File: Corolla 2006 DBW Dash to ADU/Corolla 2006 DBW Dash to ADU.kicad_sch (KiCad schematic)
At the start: 5 parts

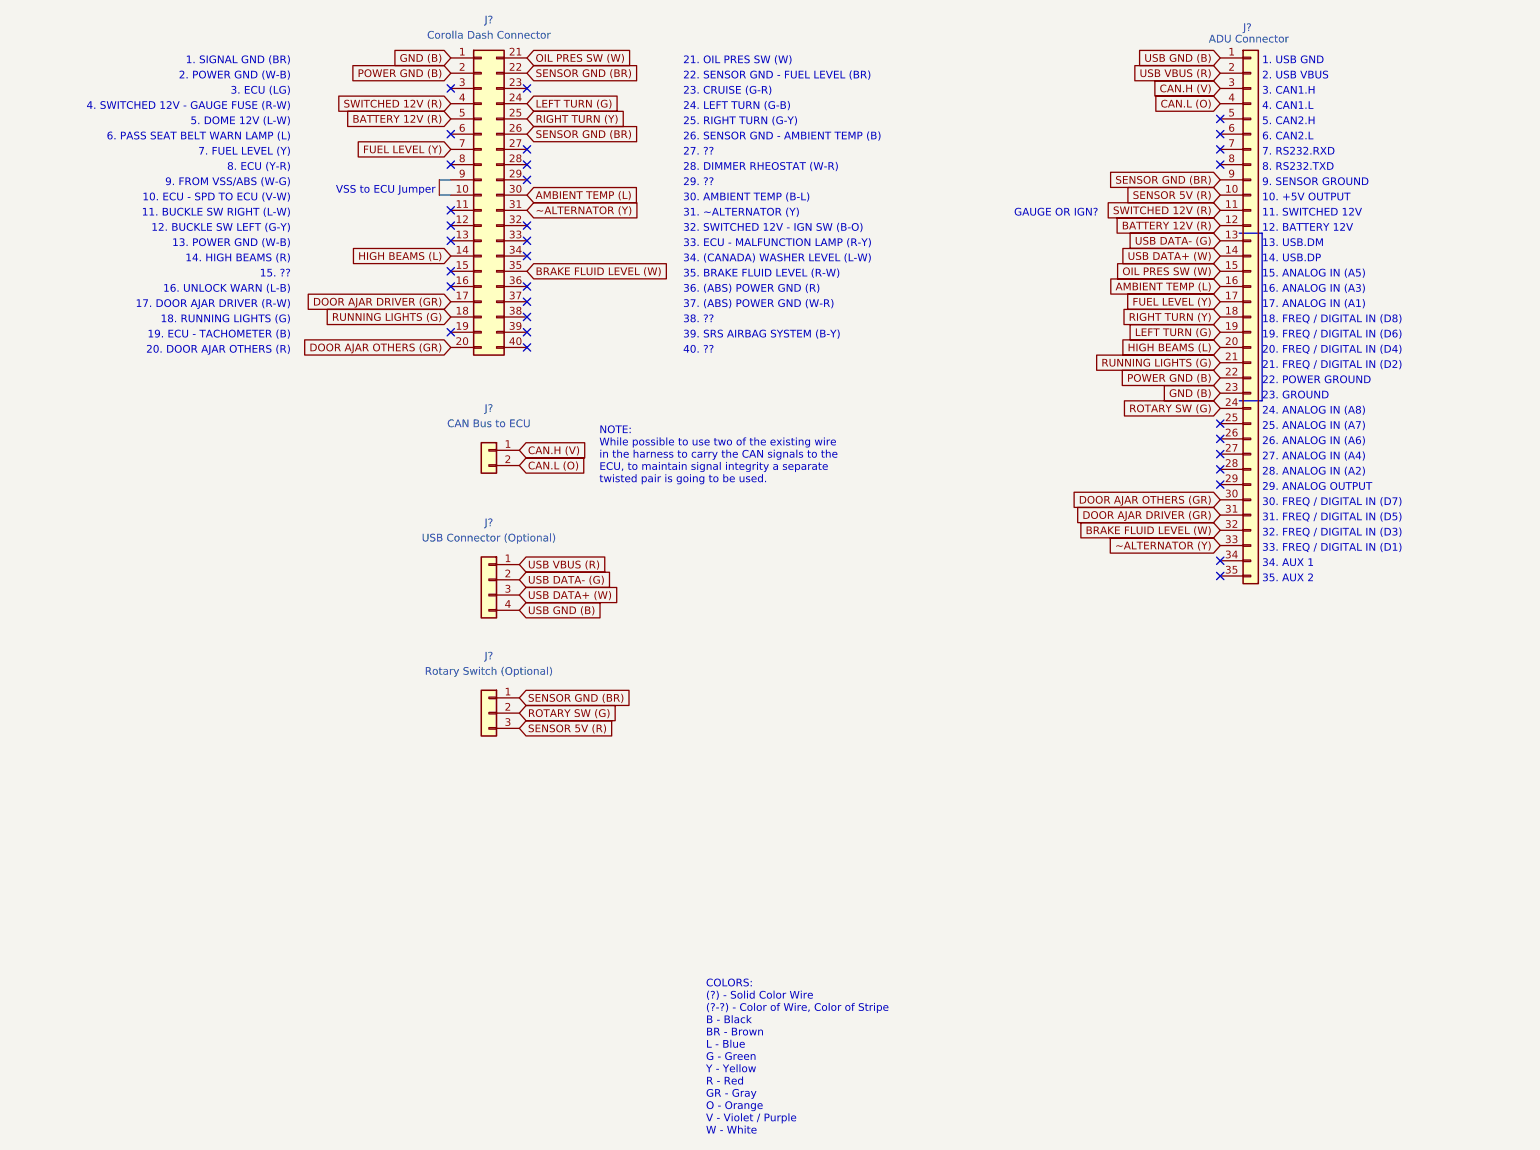
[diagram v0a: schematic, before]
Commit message: Now have a PCB to try.
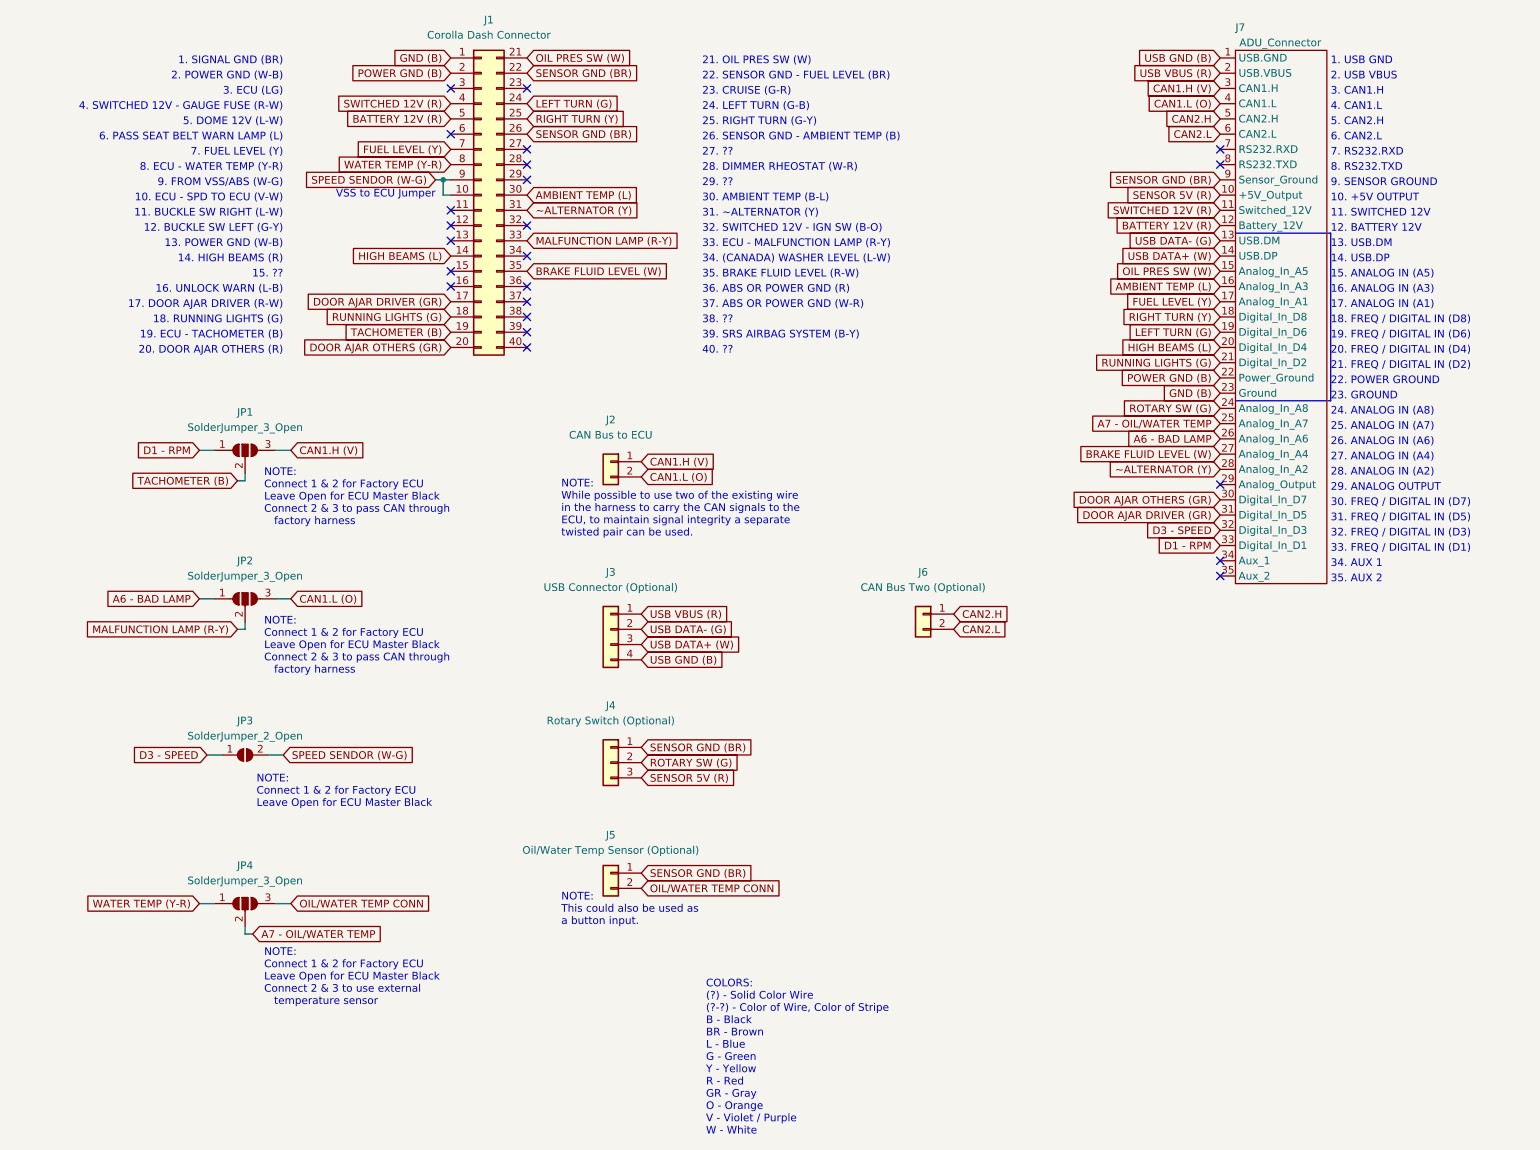
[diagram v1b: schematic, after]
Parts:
- removed J?: ADU Connector, symbol Connector_Generic:Conn_01x35
- added J5: Oil/Water Temp Sensor (Optional), Connector_Wire:SolderWire-0.75sqmm_1x02_P4.8mm_D1.25mm_OD2.3mm_Relief, symbol Connector_Generic:Conn_01x02
- added J6: CAN Bus Two (Optional), Connector_Wire:SolderWire-0.75sqmm_1x02_P4.8mm_D1.25mm_OD2.3mm_Relief, symbol Connector_Generic:Conn_01x02
- added J7: ADU_Connector, ecumaster:Wires for ADU Connector, symbol ecu_masters:ADU_Connector
- added JP1, JP2, JP4: SolderJumper_3_Open, Jumper:SolderJumper-3_P1.3mm_Open_RoundedPad1.0x1.5mm_NumberLabels, symbol Jumper:SolderJumper_3_Open
- added JP3: SolderJumper_2_Open, Jumper:SolderJumper-2_P1.3mm_Open_RoundedPad1.0x1.5mm, symbol Jumper:SolderJumper_2_Open
- J1: renamed from J?; footprint (none) -> toyota:2006 Corolla Dash Connector
- J2: renamed from J?; footprint (none) -> Connector_Wire:SolderWire-0.75sqmm_1x02_P4.8mm_D1.25mm_OD2.3mm_Relief
- J3: renamed from J?; footprint (none) -> Connector_Wire:SolderWire-0.25sqmm_1x04_P4.2mm_D0.65mm_OD1.7mm_Relief
- J4: renamed from J?; footprint (none) -> Connector_Wire:SolderWire-0.75sqmm_1x03_P4.8mm_D1.25mm_OD2.3mm_Relief
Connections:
- net AMBIENT TEMP (L): now also J7.16 (Analog_In_A3)
- net BATTERY 12V (R): now also J7.12 (Battery_12V)
- net BRAKE FLUID LEVEL (W): now also J7.27 (Analog_In_A4)
- net DOOR AJAR DRIVER (GR): now also J7.31 (Digital_In_D5)
- net DOOR AJAR OTHERS (GR): now also J7.30 (Digital_In_D7)
- net FUEL LEVEL (Y): now also J7.17 (Analog_In_A1)
- net GND (B): now also J7.23 (Ground)
- net HIGH BEAMS (L): now also J7.20 (Digital_In_D4)
- net LEFT TURN (G): now also J7.19 (Digital_In_D6)
- net OIL PRES SW (W): now also J7.15 (Analog_In_A5)
- net POWER GND (B): now also J7.22 (Power_Ground)
- net RIGHT TURN (Y): now also J7.18 (Digital_In_D8)
- net ROTARY SW (G): now also J7.24 (Analog_In_A8)
- net RUNNING LIGHTS (G): now also J7.21 (Digital_In_D2)
- net SENSOR 5V (R): now also J7.10 (+5V_Output)
- net SENSOR GND (BR): now also J5.1 (Pin_1), J7.9 (Sensor_Ground)
- net SWITCHED 12V (R): now also J7.11 (Switched_12V)
- net USB DATA+ (W): now also J7.14 (USB.DP)
- net USB DATA- (G): now also J7.13 (USB.DM)
- net USB GND (B): now also J7.1 (USB.GND)
- net USB VBUS (R): now also J7.2 (USB.VBUS)
- net ~ALTERNATOR (Y): now also J7.28 (Analog_In_A2)
- net SPEED SENDOR (W-G): now reaches J1.10 (Pin_10), J1.9 (Pin_9)
- net SPEED SENDOR (W-G): now also JP3.2 (B)
- net TACHOMETER (B): now reaches J1.19 (Pin_19)
- net TACHOMETER (B): now also JP1.2 (C)
- net MALFUNCTION LAMP (R-Y): now reaches J1.33 (Pin_33)
- net MALFUNCTION LAMP (R-Y): now also JP2.2 (C)
- net WATER TEMP (Y-R): now reaches J1.8 (Pin_8)
- net WATER TEMP (Y-R): now also JP4.1 (A)
- net CAN.H (V) renamed CAN1.H (V)
- net CAN1.H (V): now also J7.3 (CAN1.H), JP1.3 (B)
- net CAN.L (O) renamed CAN1.L (O)
- net CAN1.L (O): now also J7.4 (CAN1.L), JP2.3 (B)
- new net A6 - BAD LAMP: J7.26 (Analog_In_A6), JP2.1 (A)
- new net A7 - OIL/WATER TEMP: J7.25 (Analog_In_A7), JP4.2 (C)
- new net CAN2.H: J6.1 (Pin_1), J7.5 (CAN2.H)
- new net CAN2.L: J6.2 (Pin_2), J7.6 (CAN2.L)
- new net D1 - RPM: J7.33 (Digital_In_D1), JP1.1 (A)
- new net D3 - SPEED: J7.32 (Digital_In_D3), JP3.1 (A)
- new net OIL/WATER TEMP CONN: J5.2 (Pin_2), JP4.3 (B)
- no-connect marks 32 -> 23
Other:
- note added: "36. ABS OR POWER GND (R)"
- note added: "37. ABS OR POWER GND (W-R)"
- note added: "8. ECU - WATER TEMP (Y-R)"
- note added: "NOTE: Connect 1 & 2 for Factory ECU Leave Open for ECU Master Black"
- note added: "NOTE: Connect 1 & 2 for Factory ECU Leave Open for ECU Master Black Connect 2 & 3 to pass CAN through factory harness"
- note added: "NOTE: Connect 1 & 2 for Factory ECU Leave Open for ECU Master Black Connect 2 & 3 to use external temperature sensor"
- note added: "NOTE: This could also be used as a button input."
- note added: "NOTE: While possible to use two of the existing wire in the harness to carry the CAN signals to the ECU, to maintain signal integrity a separate twisted pair can be used."
- note removed: "36. (ABS) POWER GND (R)"
- note removed: "37. (ABS) POWER GND (W-R)"
- note removed: "8. ECU (Y-R)"
- note removed: "GAUGE OR IGN?"
- note removed: "NOTE: While possible to use two of the existing wire in the harness to carry the CAN signals to the ECU, to maintain signal integrity a separate twisted pair is going to be used."
- company: DadBodCarMod, LLC -> DadBodCarMod LLC
- title: Corolla 2006 DBW Dash to ADU Adapter -> Corolla 9th Gen ADU Dash Connector
- moved on the sheet: J2, J3, J4
